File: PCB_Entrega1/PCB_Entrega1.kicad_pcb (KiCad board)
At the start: 2 copper layers, 162.2 x 69.2 mm, 26 parts, among them J1 Conn_01x02_Male, J2 Conn_01x02_Male, T1 2N3904, T1_c1 2N3904, T1_paso1 BD135, T2 2N3904, T2_c1 2N3904, T2_paso1 BD136, T3 2N3906, T3_c1 2N3904, T4 2N3906, T4_c1 2N3904, T5_fb1 2N3904, U1 TL431D

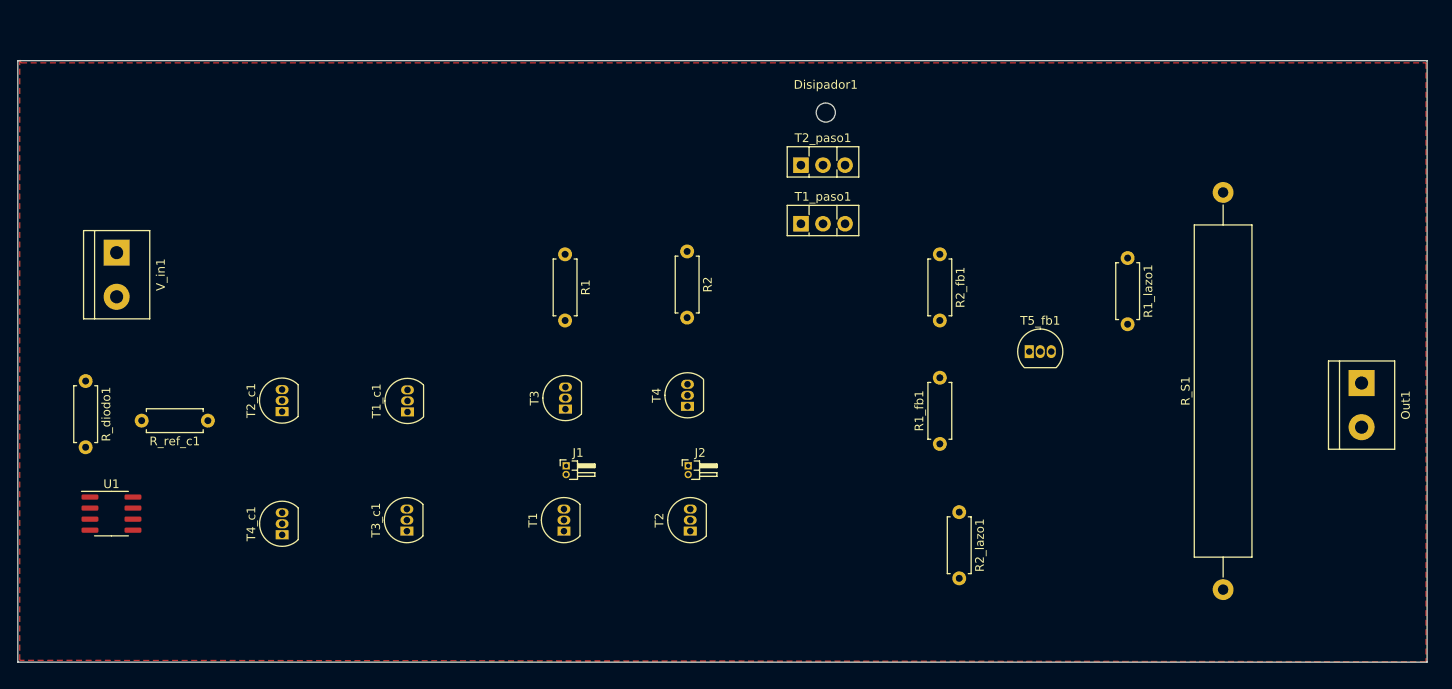
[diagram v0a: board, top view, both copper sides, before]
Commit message: PCB Checkpoint 2
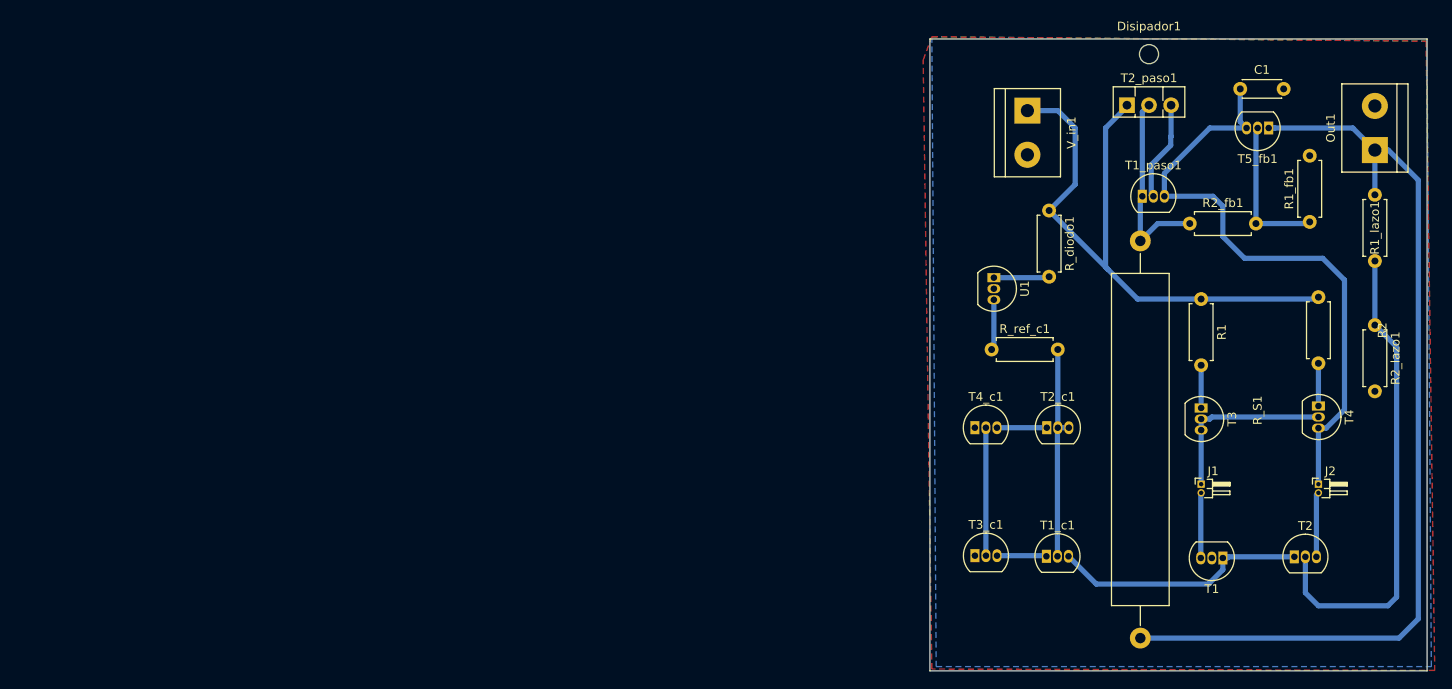
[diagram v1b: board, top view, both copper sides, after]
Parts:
- added C1: 68n, Capacitor_THT:C_Disc_D4.3mm_W1.9mm_P5.00mm, F.Cu at (227.5, 85.0)
- T1_paso1: value BD135 -> 2N3906; footprint Package_TO_SOT_THT:TO-126-3_Vertical -> Package_TO_SOT_THT:TO-92_Inline
- T2_paso1: value BD136 -> TIP32C
- U1: footprint Package_SO:SOIC-8_3.9x4.9mm_P1.27mm -> Package_TO_SOT_THT:TO-92_Inline
- moved R_diodo1 112.6 mm to (205.5, 99.0)
- moved V_in1 106.1 mm to (203.0, 87.5)
- moved U1 105.1 mm to (199.1, 106.7), turned to -90 degrees
- moved R_ref_c1 90.6 mm to (198.9, 115.0), turned to 0 degrees
- moved T2_c1 88.0 mm to (205.2, 124.0), turned to 0 degrees
- moved T4_c1 80.7 mm to (196.9, 124.0), turned to 0 degrees
- moved T1 75.9 mm to (225.5, 139.0), turned to 180 degrees
- moved T1_c1 75.4 mm to (205.2, 138.8), turned to 0 degrees
- moved R1 73.4 mm to (223.0, 109.2)
- moved T3 73.2 mm to (223.0, 121.7), turned to -90 degrees
- moved J1 73.1 mm to (223.0, 130.5)
- moved R2 72.9 mm to (236.5, 109.0)
- moved T4 72.6 mm to (236.5, 121.5), turned to -90 degrees
- moved J2 72.6 mm to (236.5, 130.5)
- moved T2 69.6 mm to (233.7, 138.9), turned to 0 degrees
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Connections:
- T1 pad 2: Net-(T1-Pad2) -> Net-(T1-B)
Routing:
- net Net-(Out1-Pin_1): track 0.00 -> 109.2 mm
- net Net-(T2_paso1-E): track 0.00 -> 72.4 mm
- net Net-(J2-Pin_1): track 0.00 -> 71.1 mm
- net Net-(T2-B): track 0.00 -> 55.4 mm
- net Net-(T1-E): track 0.00 -> 29.4 mm
- net Net-(T1_c1-B): track 0.00 -> 25.4 mm
- net Net-(T1_paso1-E): track 0.00 -> 23.0 mm
- net Net-(J1-Pin_1): track 0.00 -> 21.1 mm
- net Net-(T2_c1-E): track 0.00 -> 20.5 mm
- net Net-(T5_fb1-B): track 0.00 -> 17.3 mm
- net Net-(T1_paso1-C): track 0.00 -> 11.6 mm
- net Net-(J1-Pin_2): track 0.00 -> 7.52 mm
- net Net-(J2-Pin_2): track 0.00 -> 7.46 mm
- net Net-(U1-K): track 0.00 -> 6.41 mm
- net Net-(R_ref_c1-Pad1): track 0.00 -> 5.84 mm
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- added copper zone on B.Cu, net GND
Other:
- board size 162.2 x 69.2 mm -> 57.2 x 72.7 mm
